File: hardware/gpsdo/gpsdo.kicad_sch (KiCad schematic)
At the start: 19 parts, among them U1 74HC4040D_652, U2 74HC4040D_652, U3 AD5693RxRM, U4 PCA9306

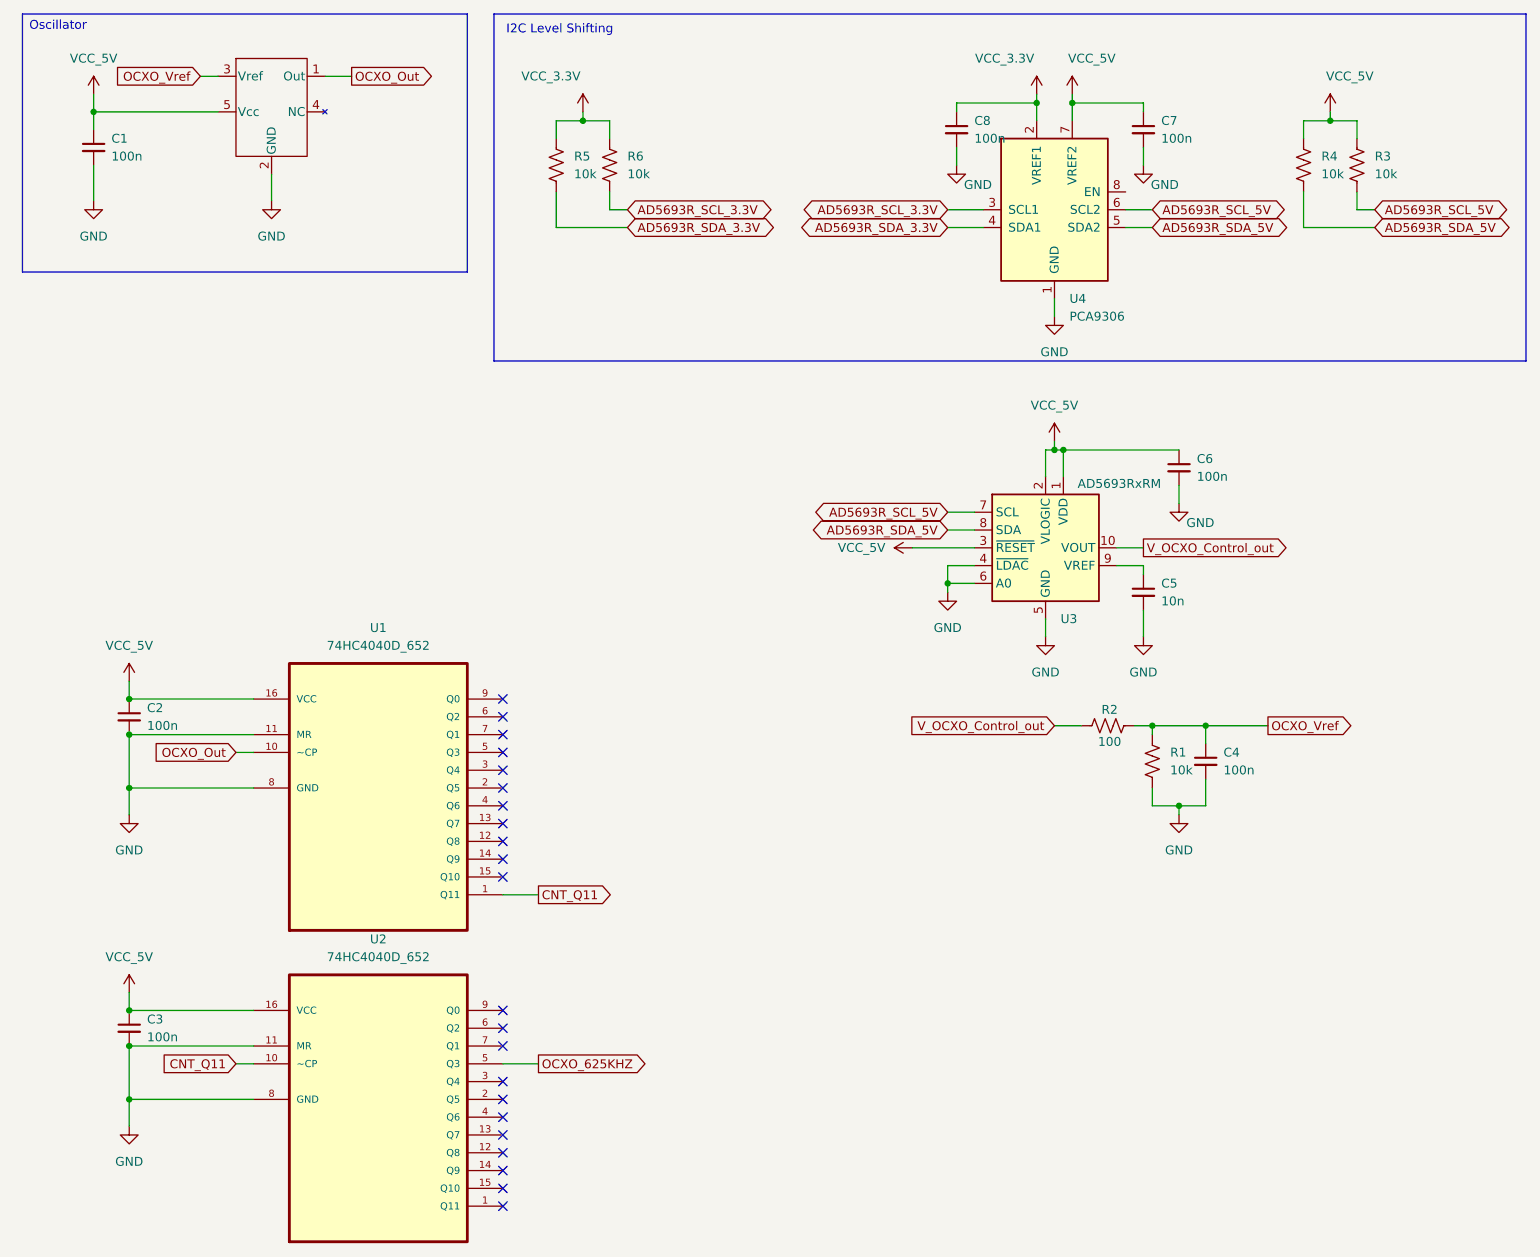
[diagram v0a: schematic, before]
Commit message: update schematics
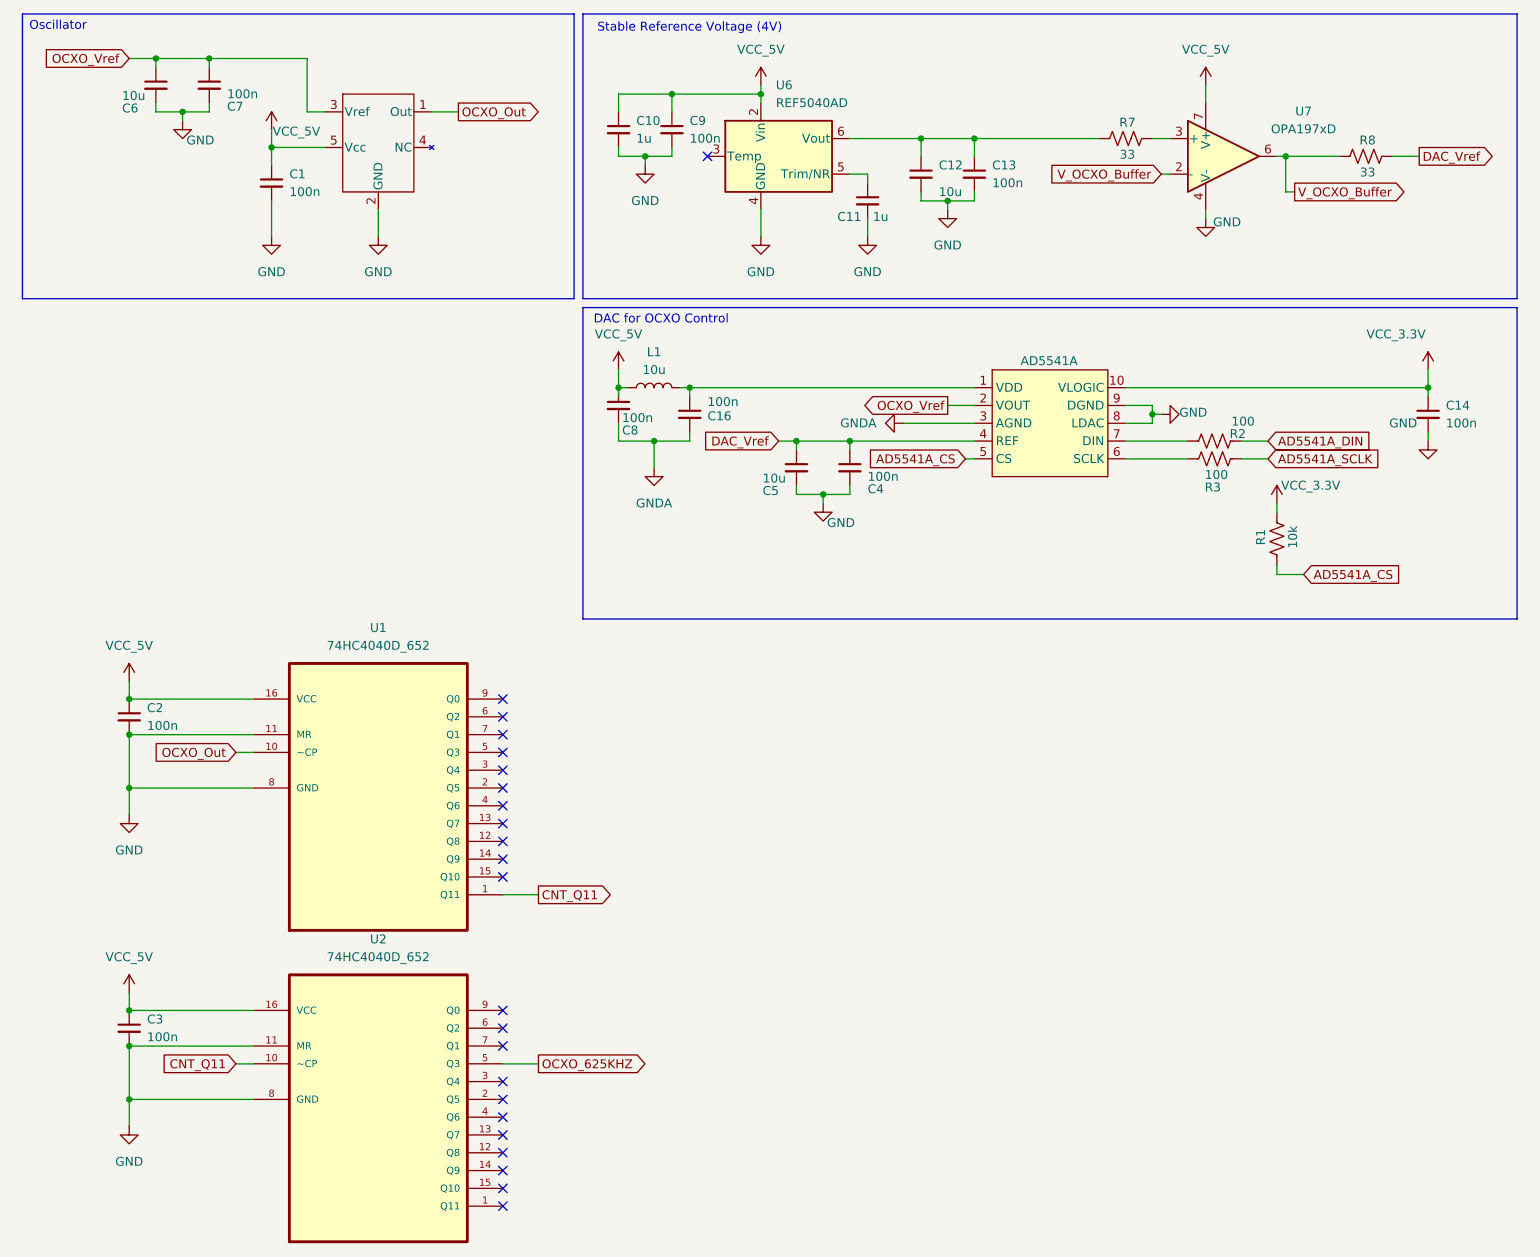
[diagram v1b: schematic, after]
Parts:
- removed R4, R5, R6: 10k, Resistor_SMD:R_0201_0603Metric_Pad0.64x0.40mm_HandSolder, symbol Device:R_US
- removed U3: AD5693RxRM, Package_SO:MSOP-10_3x3mm_P0.5mm, symbol Analog_DAC:AD5693RxRM
- removed U4: PCA9306, symbol Interface:PCA9306
- added AD5541A: ~, symbol AD5541A:AD5541A
- added C10, C11: 1u, Capacitor_SMD:C_0201_0603Metric_Pad0.64x0.40mm_HandSolder, symbol Device:C_Small
- added C12: 10u, Capacitor_SMD:C_0201_0603Metric_Pad0.64x0.40mm_HandSolder, symbol Device:C_Small
- added C13, C14, C16, C9: 100n, Capacitor_SMD:C_0201_0603Metric_Pad0.64x0.40mm_HandSolder, symbol Device:C_Small
- added L1: 10u, Capacitor_SMD:C_0201_0603Metric_Pad0.64x0.40mm_HandSolder, symbol Device:L
- added R7, R8: 33, Resistor_SMD:R_0201_0603Metric_Pad0.64x0.40mm_HandSolder, symbol Device:R_US
- added U6: REF5040AD, Package_SO:SOIC-8_3.9x4.9mm_P1.27mm, symbol Reference_Voltage:REF5040AD
- added U7: OPA197xD, Package_SO:SOIC-8_3.9x4.9mm_P1.27mm, symbol Amplifier_Operational:OPA197xD
- C5: value 10n -> 10u
- C6: value 100n -> 10u
- R3: value 10k -> 100
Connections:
- net GND: now also AD5541A.8 (LDAC), AD5541A.9 (DGND), C10.2, C11.2, C12.2, C13.2, C14.2, C9.2, U6.4 (GND), U7.4 (V-); no longer C8.2, R1.2
- net OCXO_Vref: now also C6.1, C7.1, AD5541A.2 (VOUT); no longer C4.1, R1.1, R2.2
- net VCC_3.3V: now also R1.2, AD5541A.10 (VLOGIC), C14.1; no longer C8.1
- net VCC_5V: now also C8.1, C10.1, C9.1, L1.1, U6.2 (Vin), U7.7 (V+); no longer C6.1, C7.1, R3.1
- net DAC_Vref: now reaches C5.1
- net DAC_Vref: now also C4.1, AD5541A.4 (REF), R8.2
- net AD5693R_SCL_5V renamed AD5541A_SCLK
- net V_OCXO_Control_out: no longer names the net of R2.1
- net V_OCXO_Control_out: now also AD5541A.7 (DIN)
- new net: C12.1, C13.1, R7.1, U6.6 (Vout)
- new net: C11.1, U6.5 (Trim/NR)
- new net: R7.2, U7.3 (+)
- new net: AD5541A.6 (SCLK), R3.1
- new net: AD5541A.1 (VDD), C16.1, L1.2
- new net AD5541A_CS: AD5541A.5 (CS), R1.1
- new net AD5541A_DIN: R2.2
- new net GNDA: AD5541A.3 (AGND), C16.2, C8.2
- new net V_OCXO_Buffer: R8.1, U7.2 (-), U7.6
- no-connect marks 22 -> 23
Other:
- note added: "DAC for OCXO Control"
- note added: "Stable Reference Voltage (4V)"
- note removed: "I2C Level Shifting"
- moved on the sheet: C1, C4
